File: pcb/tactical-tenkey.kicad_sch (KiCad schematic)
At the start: 42 parts, among them Q1 FS8205A, SW1 SW_SPST, U1 XIAO-ESP32-S3-SMD, U2 DW01A

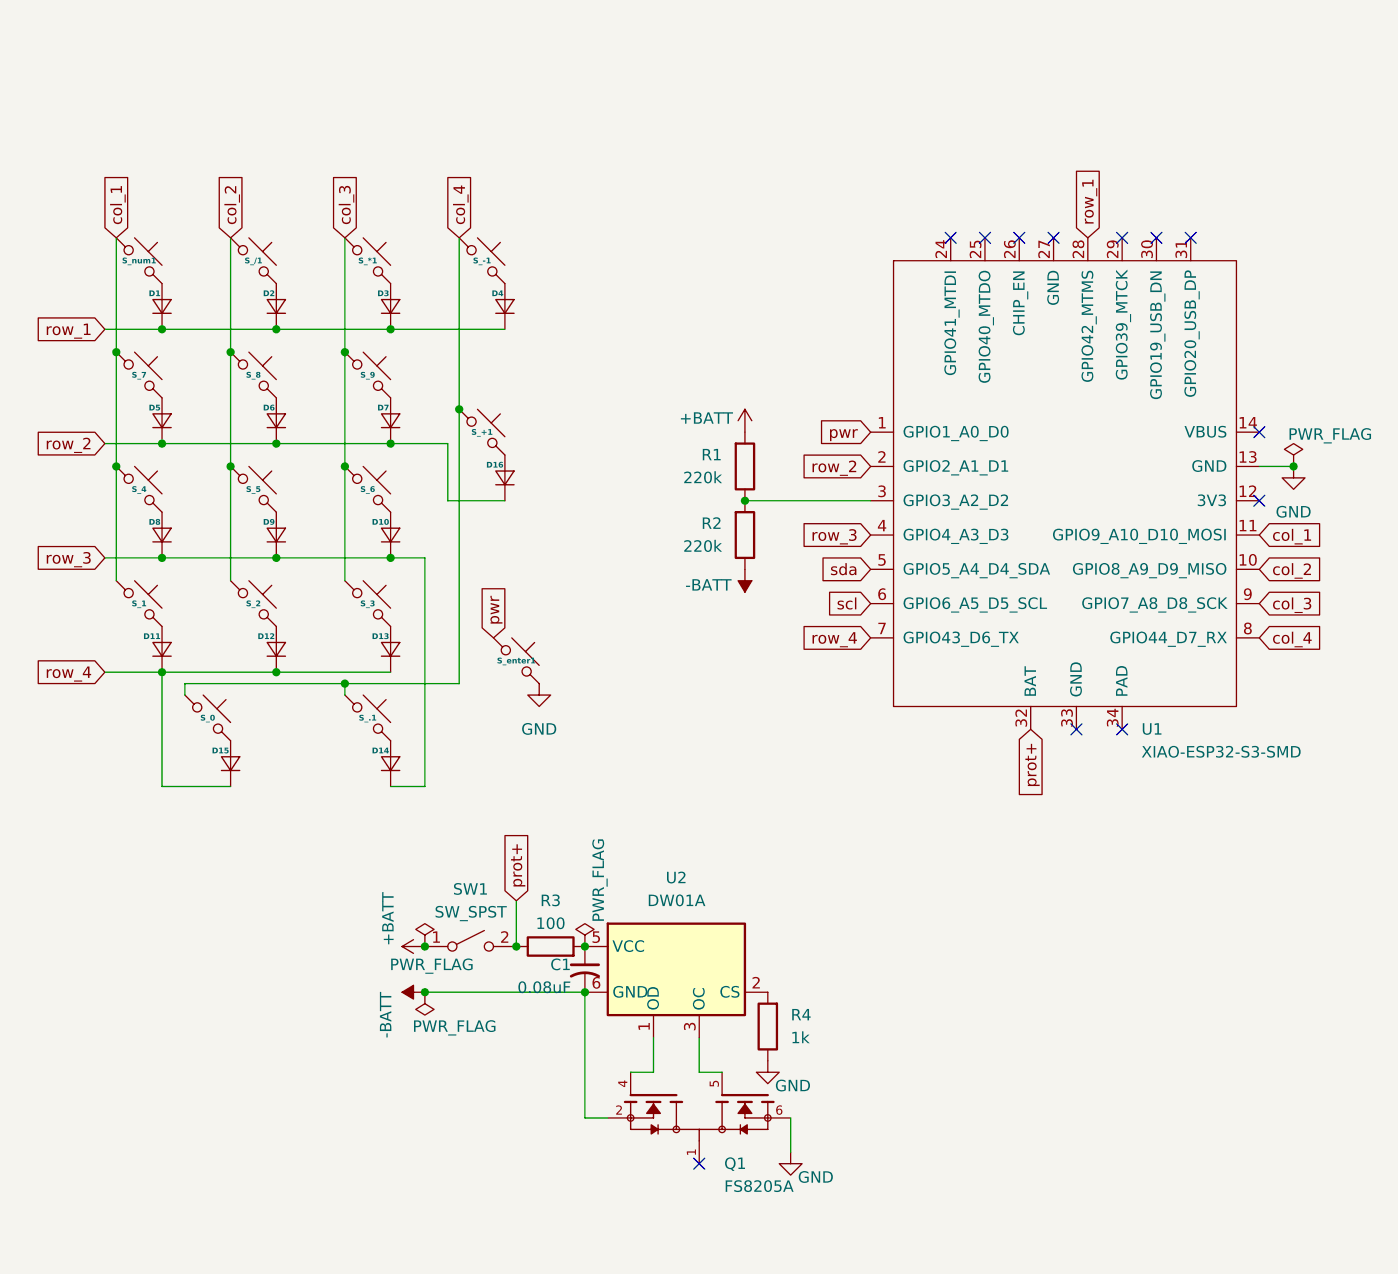
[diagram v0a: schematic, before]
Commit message: pcb layout
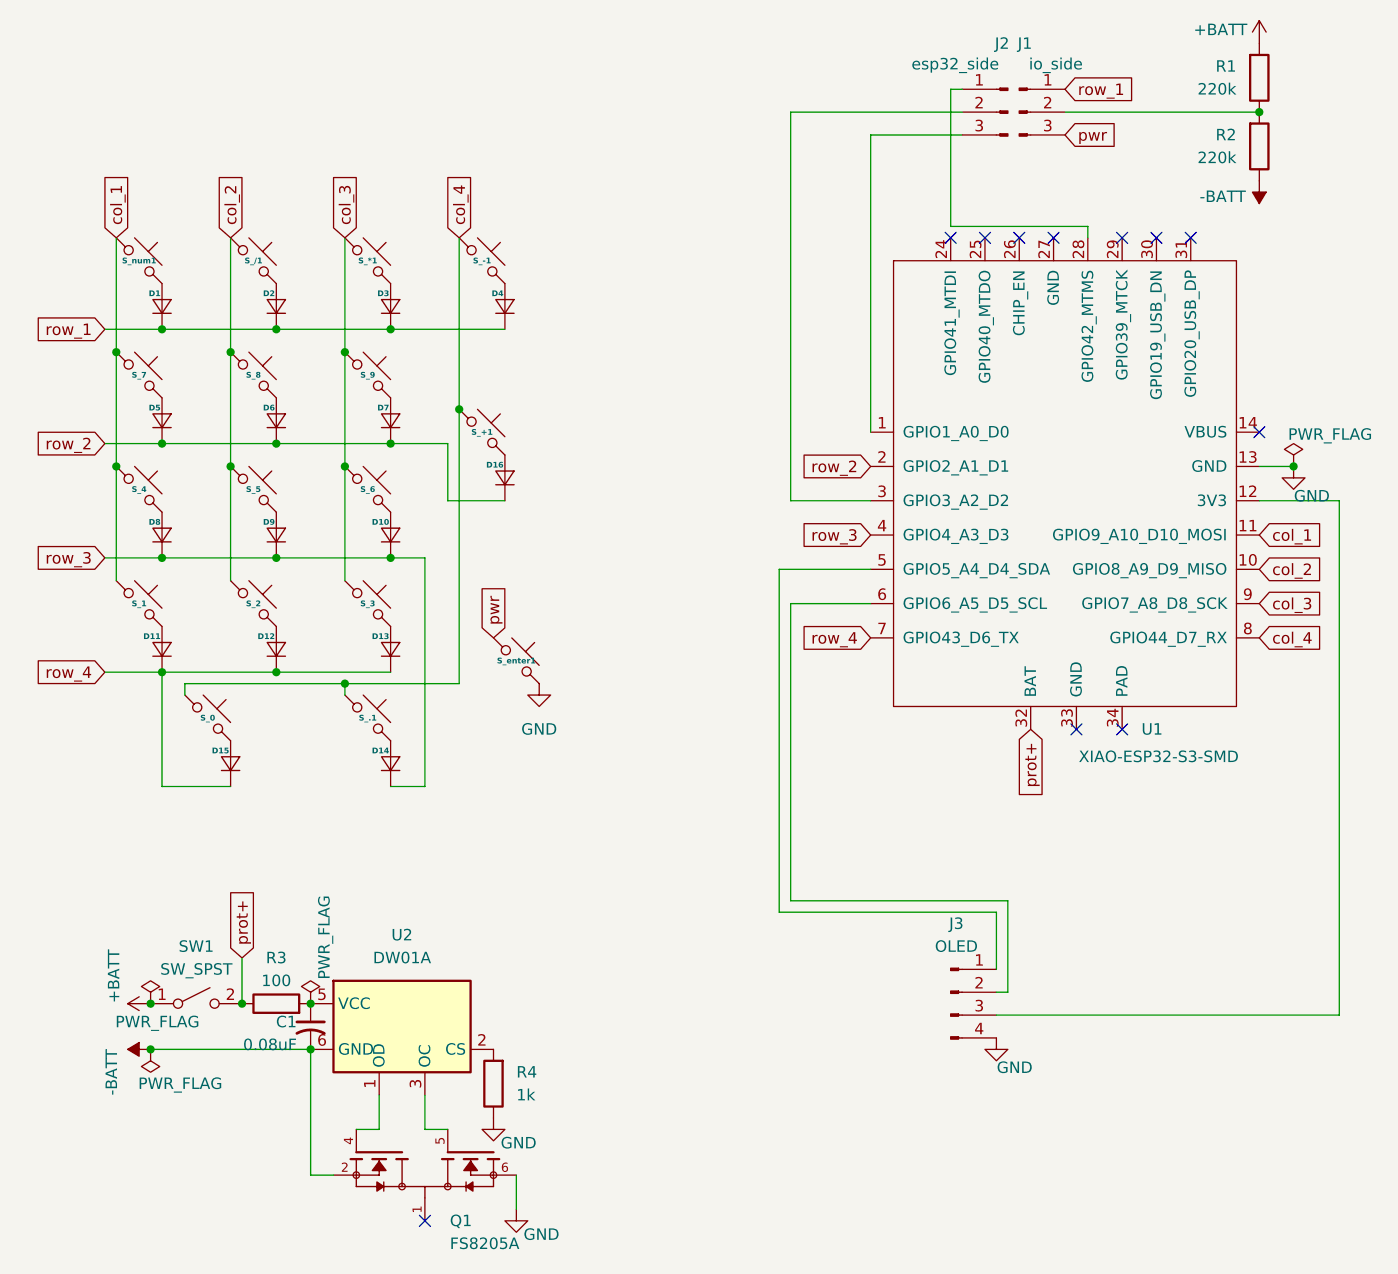
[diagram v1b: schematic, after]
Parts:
- added J1: io_side, Connector_PinHeader_2.54mm:PinHeader_1x03_P2.54mm_Vertical, symbol Connector:Conn_01x03_Pin
- added J2: esp32_side, Connector_PinHeader_2.54mm:PinHeader_1x03_P2.54mm_Vertical, symbol Connector:Conn_01x03_Pin
- added J3: OLED, Connector_PinHeader_2.54mm:PinHeader_1x04_P2.54mm_Vertical, symbol Connector:Conn_01x04_Pin
- C1: footprint (none) -> Capacitor_THT:CP_Radial_Tantal_D4.5mm_P5.00mm
- D1, D10, D11, D12, D13, D14, D15, D16, D2, D3, D4, D5, D6, D7, D8, D9: footprint (none) -> ScottoKeebs_Components:Diode_DO-35
- R1, R2, R3, R4: footprint (none) -> Resistor_THT:R_Axial_DIN0207_L6.3mm_D2.5mm_P10.16mm_Horizontal
- SW1: footprint (none) -> Button_Switch_THT:SW_SPST_Omron_B3F-315x_Angled
- S_*1, S_-1, S_.1, S_/1, S_1, S_2, S_3, S_4, S_5, S_6, S_7, S_8, S_9: footprint (none) -> ScottoKeebs_MX:MX_PCB_1.00u
- S_+1, S_enter1: footprint (none) -> ScottoKeebs_MX:MX_PCB_2.00u_90deg
- S_0: footprint (none) -> ScottoKeebs_MX:MX_PCB_2.00u
- S_num1: footprint (none) -> ScottoKeebs_MX:MX_PCB
- U1: footprint Seeed_Studio_XIAO_Series:XIAO-ESP32-S3-SMD -> xiao:XIAO-ESP32-S3-SMD_PAD
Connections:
- net GND: now also J3.4 (Pin_4)
- net pwr: now also J1.3 (Pin_3); no longer U1.1 (GPIO1_A0_D0)
- net row_1: now also J1.1 (Pin_1); no longer U1.28 (GPIO42_MTMS)
- net at U1.12 (3V3): now also J3.3 (Pin_3)
- net at R1.1, R2.2: now also J1.2 (Pin_2); no longer U1.3 (GPIO3_A2_D2)
- net scl: no longer names the net of U1.6 (GPIO6_A5_D5_SCL)
- net scl: now also J3.2 (Pin_2)
- net sda: no longer names the net of U1.5 (GPIO5_A4_D4_SDA)
- net sda: now also J3.1 (Pin_1)
- new net: J2.3 (Pin_3), U1.1 (GPIO1_A0_D0)
- new net: J2.1 (Pin_1), U1.28 (GPIO42_MTMS)
- new net: J2.2 (Pin_2), U1.3 (GPIO3_A2_D2)
- no-connect marks 12 -> 11
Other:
- moved on the sheet: C1, Q1, R1, R2, R3, R4, SW1, U2
